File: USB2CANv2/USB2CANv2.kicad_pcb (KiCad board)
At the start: 4 copper layers, 48.6 x 20.3 mm, 64 parts, among them IC1 MIC5528-3.3YMT-TR, J1 USB_C_Receptacle_USB2.0, J2 Conn_01x06_Pin, J3 Conn_01x02_Pin, J4 Conn_01x02_Pin, J5 Conn_01x02_Pin, SW1 SW_BOOT0, U1 STM32F405RGTx, U2 USBLC6-2P6, U3 MCP2561-E-SN, U4 TLP175A, U5 MCP2561-E-SN, U6 TLP175A, Y1 16MHz, Y2 32KHz

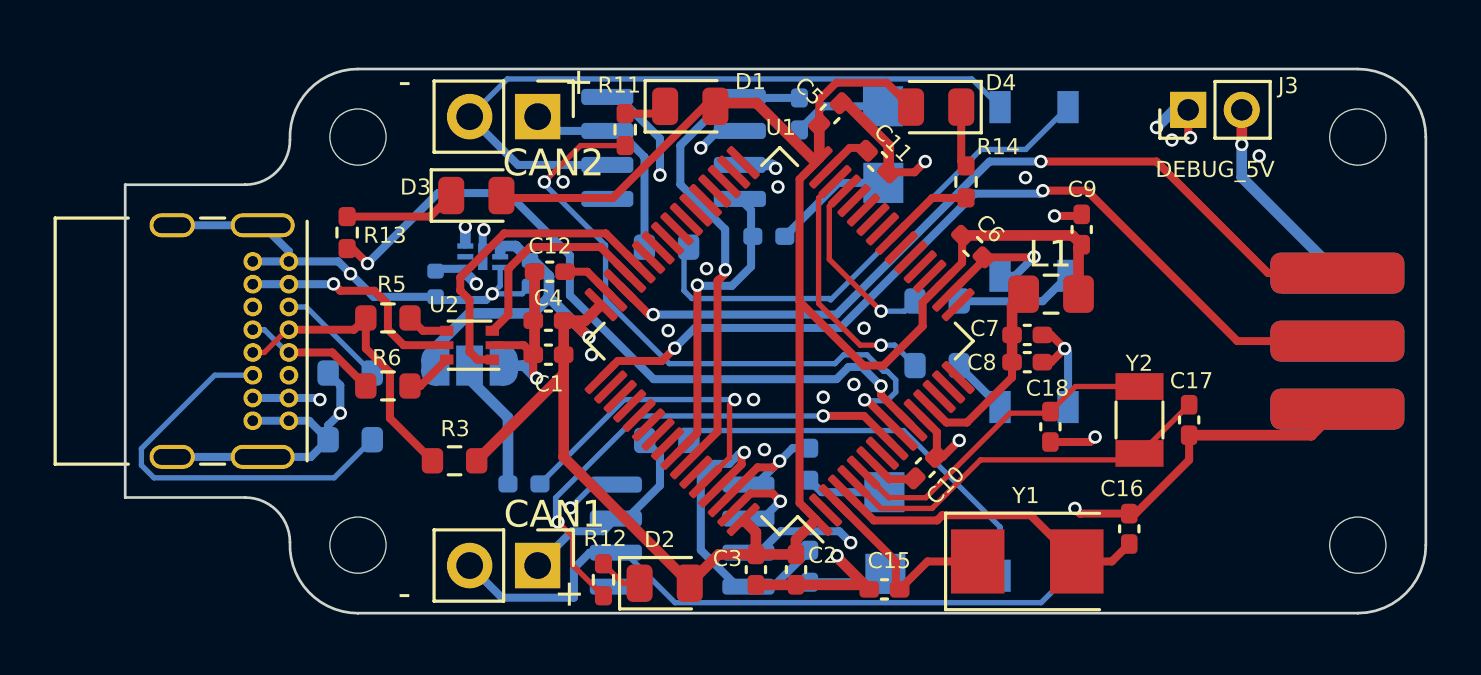
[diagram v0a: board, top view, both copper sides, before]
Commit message: Board done
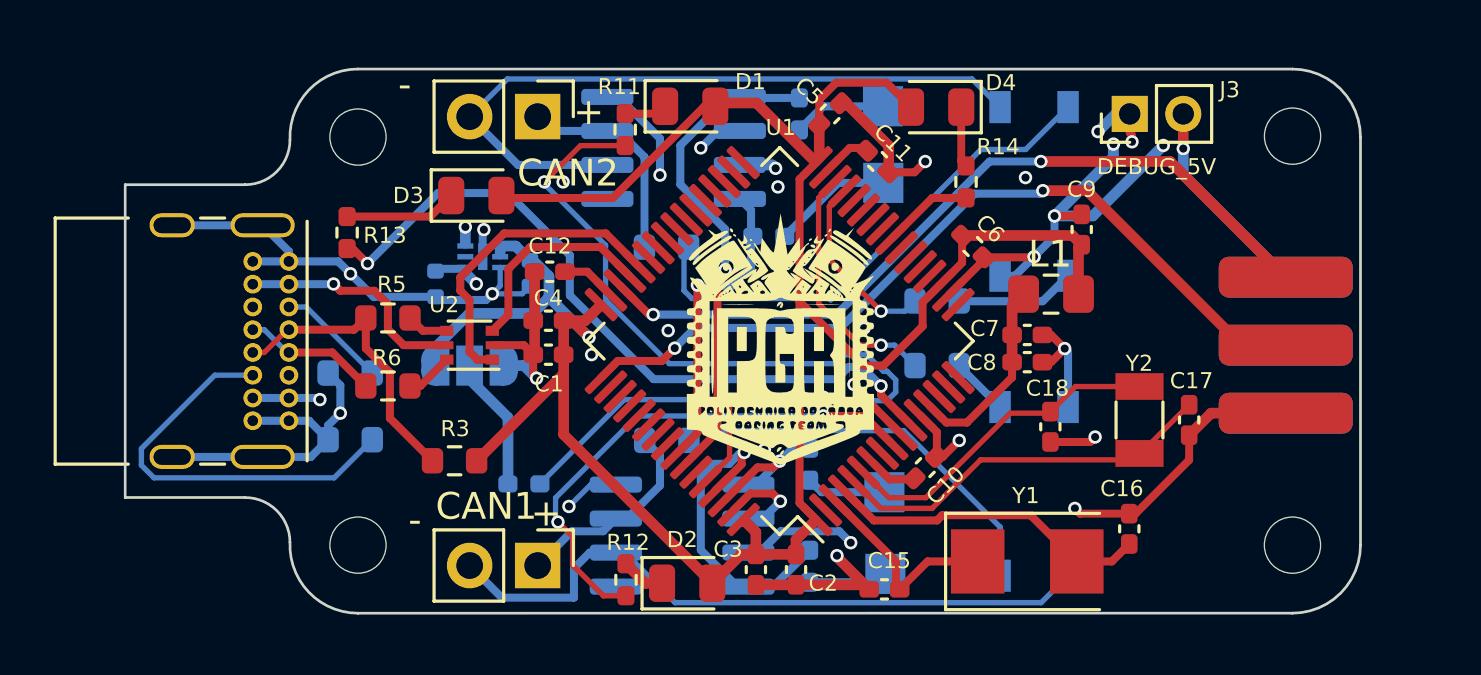
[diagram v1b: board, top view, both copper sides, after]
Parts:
- added G***: LOGO, footprints:PGR_srednie, F.Cu at (145.4, 97.6)
- added G***: LOGO, footprints:PGR_male, B.Cu at (144.3, 98.0)
- moved H3 2.44 mm to (164.6, 105.3)
- moved H4 2.44 mm to (164.6, 90.0)
- moved J3 2.19 mm to (158.5, 89.2)
- moved J2 1.94 mm to (164.3, 97.8)
- moved D2 0.84 mm to (142.0, 106.7)
- moved R12 0.84 mm to (139.7, 106.6)
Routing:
- net GND: track 87.6 -> 96.2 mm
- net /SWCLK: track 32.7 -> 30.8 mm
- net /SWDIO: track 31.3 -> 29.5 mm
- net /DEBUG_5V: track 7.58 -> 8.98 mm
- net /LED_CAN1: track 18.7 -> 19.5 mm
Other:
- board size 48.6 x 20.3 mm -> 46.1 x 20.3 mm
- board text added: "Mieszko Celinski Karol Pergol"
- board text added: "USB2CANv2"
